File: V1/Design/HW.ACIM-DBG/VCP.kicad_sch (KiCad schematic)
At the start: 15 parts, among them J4 VCP ICSP, U4 PIC32MM0064GPM028

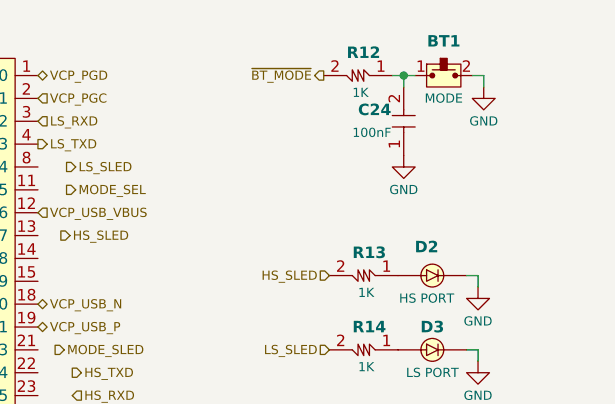
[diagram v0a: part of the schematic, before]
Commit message: V1 schematic update 3
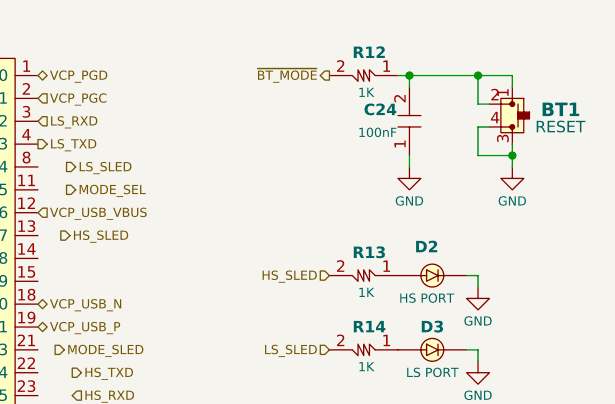
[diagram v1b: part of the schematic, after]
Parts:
- removed BT1: MODE, Liem:SW_SMD2_6.0x3.5, symbol SAMPI:BT3
- added BT1: RESET, SAMPI:BUTTON_4P_6x6, symbol SAMPI:BT
- C19, C20, C21, C24: footprint Liem:CAP0402 -> SAMPI:CAP0603; MFT Walsin Technology Corporation -> Samsung; MNP 0402B104K160CT -> CL10B104KB8NNNC
- C22, C23: footprint Liem:CAP0603 -> SAMPI:CAP0603; MFT KEMET -> Samsung; MNP C0603C106M8PACTU -> CL10A106MQ8NNNC
- D2: footprint Liem:LED0603 -> SAMPI:LED0603; MFT Rohm Semiconductor -> Harvatek; MNP SML-D12V8WT86P -> B1931NB--20C007614U1930
- D3: footprint Liem:LED0603 -> SAMPI:LED0603; MFT Rohm Semiconductor -> Harvatek; MNP SML-D12V8WT86P -> B1911NG--20D000214U1930
- J4: footprint (none) -> SAMPI:HD-1x6x1.27MM-TH; MFT <NULL> -> Harwin; MNP <NULL> -> M50-3530642
- R11: footprint Liem:RES0402 -> SAMPI:RES0603; MNP RC0402FR-0710KL -> RC0603FR-0710KL
- R12, R13, R14: footprint Liem:RES0402 -> SAMPI:RES0603; MFT Rohm Semiconductor -> YAGEO; MNP MCR01MZPJ102 -> RC0603FR-071KL
- U4: footprint Liem:UQFN28-4x4-EP -> SAMPI:UQFN28-4x4-EP
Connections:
- net GND: now also BT1.3, BT1.4
- net at C24.2, R12.1: now also BT1.1, BT1.2
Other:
- moved on the sheet: C24, R12
